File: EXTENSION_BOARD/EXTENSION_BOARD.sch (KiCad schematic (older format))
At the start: 35 parts, among them IC1 TeensyBuffer - 74AHCV541ABQX, IC2 Baro - MS561101BA03-50, J1 EXTIN, J2 BATT, J3 PWM, J4 EXTOUT, U1 Flash - COM-15809, U2 Teensy4.0, U3 MJD148J

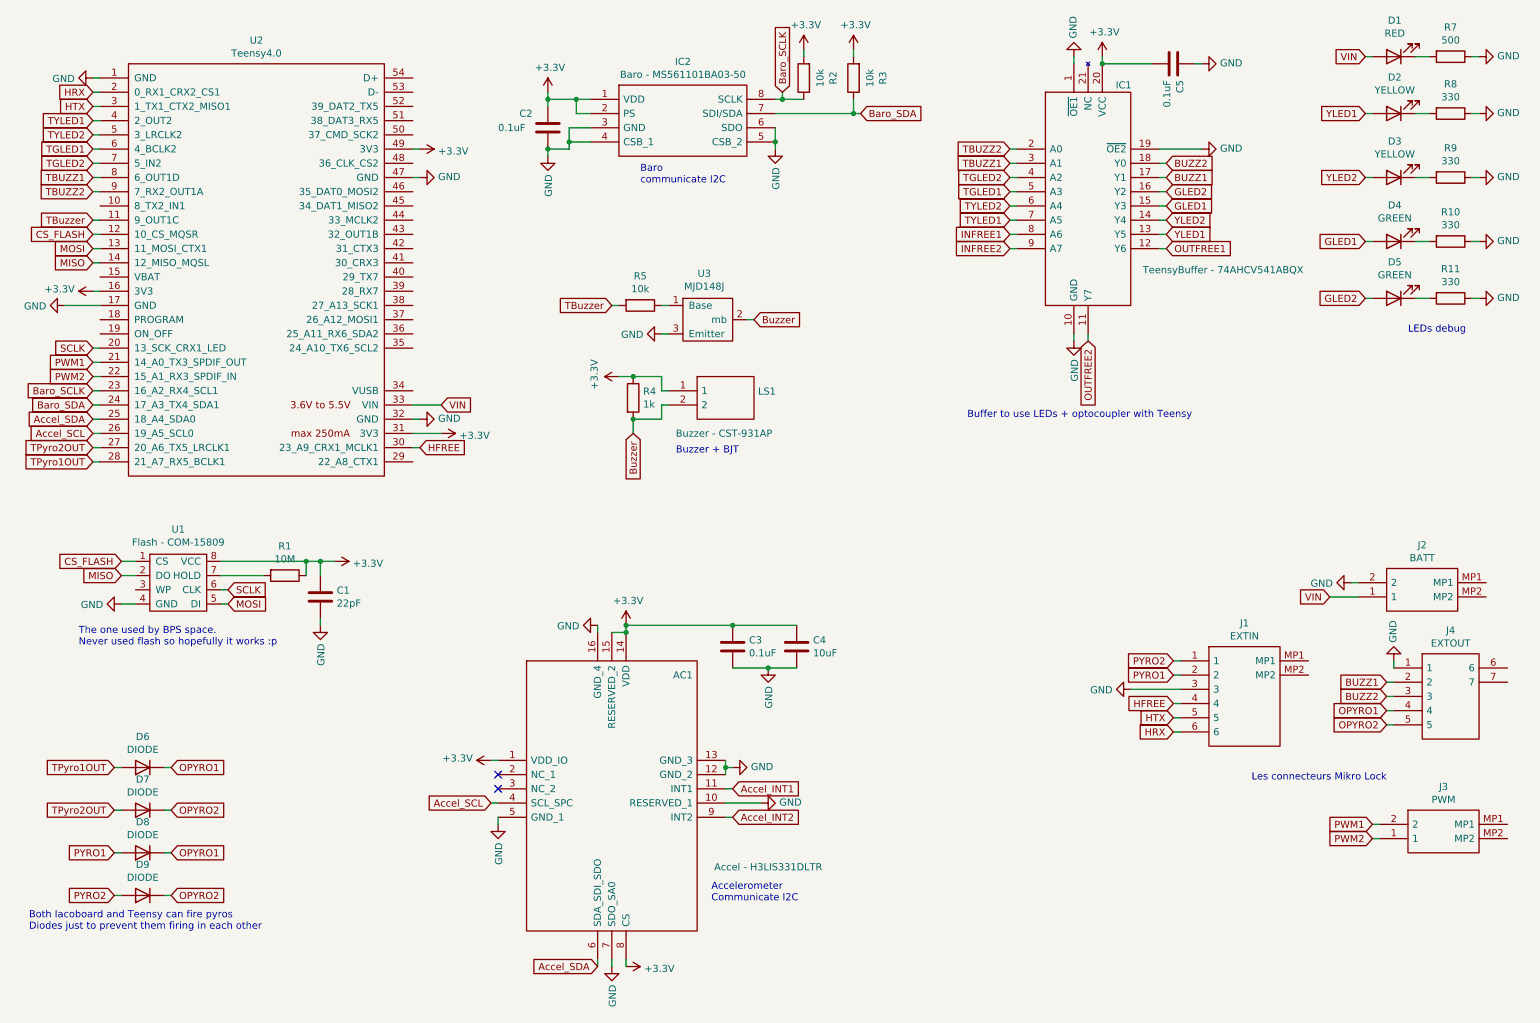
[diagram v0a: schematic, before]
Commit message: t
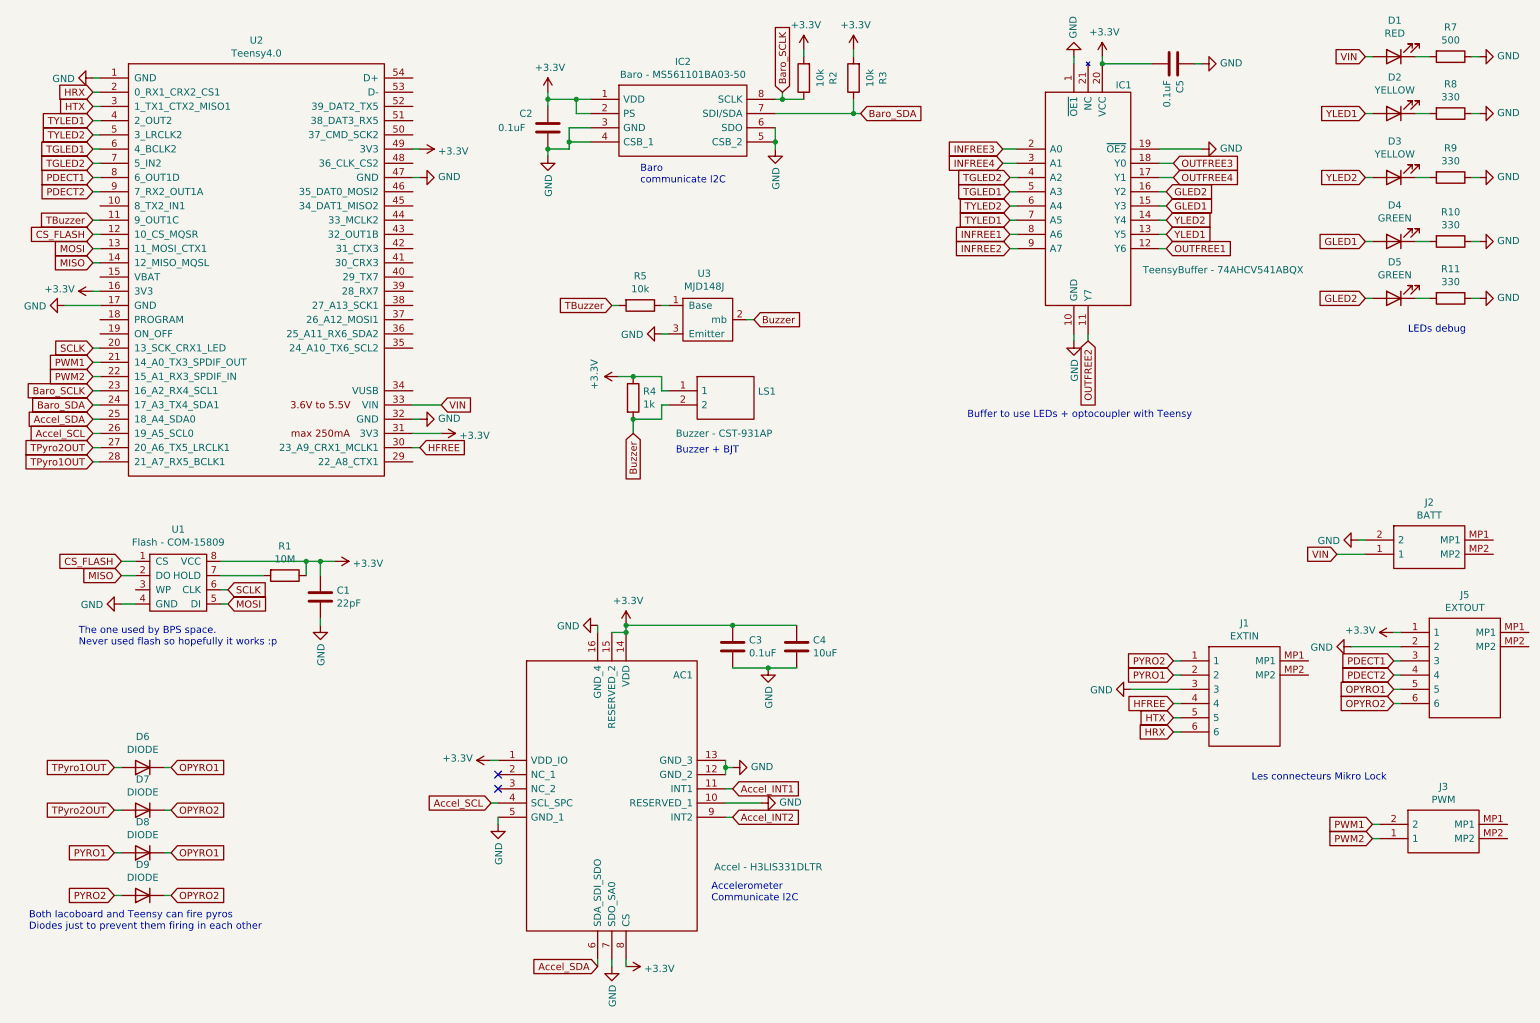
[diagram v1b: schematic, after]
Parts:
- removed J4: EXTOUT, EXTENSION:5055670571, symbol EXTENSION:505567-0571
- added J5: EXTOUT, EXTENSION:5055670671, symbol EXTENSION:505567-0671
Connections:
- net +3V3: now also J5.1
- net GND: now also J5.2
- net OPYRO1: now also J5.5
- net OPYRO2: now also J5.6
- net BUZZ1 renamed OUTFREE4
- net BUZZ2 renamed OUTFREE3
- net TBUZZ1 renamed INFREE4
- net INFREE4: no longer U2.8 (6_OUT1D)
- net TBUZZ2 renamed INFREE3
- net INFREE3: no longer U2.9 (7_RX2_OUT1A)
- new net PDECT1: J5.3, U2.8 (6_OUT1D)
- new net PDECT2: J5.4, U2.9 (7_RX2_OUT1A)
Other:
- moved on the sheet: J2
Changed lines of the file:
@@
 	3500 3450 3300 3450
-$Comp
-L EXTENSION:505567-0571 J4
-U 1 1 618D57EA
-P 10200 5100
-F 0 "J4" H 10600 5365 50  0000 C CNN
-F 1 "EXTOUT" H 10600 5274 50  0000 C CNN
-F 2 "EXTENSION:5055670571" H 10850 5200 50  0001 L CNN
-F 3 "https://www.molex.com/pdm_docs/sd/5055670571_sd.pdf" H 10850 5100 50  0001 L CNN
-F 4 "Molex Micro-Lock PLUS 505567, 1.25mm Pitch, 5 Way, 1 Row, Right Angle PCB Header, Surface Mount" H 10850 5000 50  0001 L CNN "Description"
-F 5 "3" H 10850 4900 50  0001 L CNN "Height"
-F 6 "538-505567-0571" H 10850 4800 50  0001 L CNN "Mouser Part Number"
-F 7 "https://www.mouser.co.uk/ProductDetail/Molex/505567-0571?qs=gt1LBUVyoHnJxHrzoS78pw%3D%3D" H 10850 4700 50  0001 L CNN "Mouser Price/Stock"
-F 8 "Molex" H 10850 4600 50  0001 L CNN "Manufacturer_Name"
-F 9 "505567-0571" H 10850 4500 50  0001 L CNN "Manufacturer_Part_Number"
-	1    10200 5100
-	1    0    0    -1
-$EndComp
 $Comp
 L EXTENSION:505567-0281 J3
@@
 	10050 6300 10100 6300
 $Comp
-L power:GND #PWR034
-U 1 1 618E3668
-P 10200 5050
-F 0 "#PWR034" H 10200 4800 50  0001 C CNN
-F 1 "GND" V 10205 4922 50  0000 R CNN
-F 2 "" H 10200 5050 50  0001 C CNN
-F 3 "" H 10200 5050 50  0001 C CNN
-	1    10200 5050
-	-1   0    0    1
-$EndComp
-Wire Wire Line
-	10150 5500 10200 5500
-Text GLabel 10150 5300 0    50   Input ~ 0
-BUZZ2
-Wire Wire Line
-	10150 5400 10200 5400
-Text GLabel 10150 5200 0    50   Input ~ 0
-BUZZ1
-Text GLabel 10150 5500 0    50   Input ~ 0
-OPYRO2
-Text GLabel 10150 5400 0    50   Input ~ 0
-OPYRO1
-Wire Wire Line
-	10150 5200 10200 5200
-Wire Wire Line
-	10150 5300 10200 5300
-$Comp
 L EXTENSION:505567-0281 J2
 U 1 1 61906994
-P 9950 4500
-F 0 "J2" H 10400 4765 50  0000 C CNN
-F 1 "BATT" H 10400 4674 50  0000 C CNN
-F 2 "EXTENSION:5055670281" H 10700 4600 50  0001 L CNN
-F 3 "https://www.molex.com/pdm_docs/sd/5055670281_sd.pdf" H 10700 4500 50  0001 L CNN
-F 4 "Headers & Wire Housings MicroLockPlus 1.25MM RA HDR SR 2P BLK GLD" H 10700 4400 50  0001 L CNN "Description"
-F 5 "3.9" H 10700 4300 50  0001 L CNN "Height"
-F 6 "538-505567-0281" H 10700 4200 50  0001 L CNN "Mouser Part Number"
-F 7 "https://www.mouser.co.uk/ProductDetail/Molex/505567-0281?qs=gt1LBUVyoHmc7tfcrPDm5A%3D%3D" H 10700 4100 50  0001 L CNN "Mouser Price/Stock"
-F 8 "Molex" H 10700 4000 50  0001 L CNN "Manufacturer_Name"
-F 9 "505567-0281" H 10700 3900 50  0001 L CNN "Manufacturer_Part_Number"
-	1    9950 4500
-	1    0    0    -1
-$EndComp
-Text GLabel 9750 4600 0    50   Input ~ 0
+P 10000 4200
+F 0 "J2" H 10450 4465 50  0000 C CNN
+F 1 "BATT" H 10450 4374 50  0000 C CNN
+F 2 "EXTENSION:5055670281" H 10750 4300 50  0001 L CNN
+F 3 "https://www.molex.com/pdm_docs/sd/5055670281_sd.pdf" H 10750 4200 50  0001 L CNN
+F 4 "Headers & Wire Housings MicroLockPlus 1.25MM RA HDR SR 2P BLK GLD" H 10750 4100 50  0001 L CNN "Description"
+F 5 "3.9" H 10750 4000 50  0001 L CNN "Height"
+F 6 "538-505567-0281" H 10750 3900 50  0001 L CNN "Mouser Part Number"
+F 7 "https://www.mouser.co.uk/ProductDetail/Molex/505567-0281?qs=gt1LBUVyoHmc7tfcrPDm5A%3D%3D" H 10750 3800 50  0001 L CNN "Mouser Price/Stock"
+F 8 "Molex" H 10750 3700 50  0001 L CNN "Manufacturer_Name"
+F 9 "505567-0281" H 10750 3600 50  0001 L CNN "Manufacturer_Part_Number"
+	1    10000 4200
+	1    0    0    -1
+$EndComp
+Text GLabel 9800 4300 0    50   Input ~ 0
 VIN
 Wire Wire Line
-	9900 4500 9950 4500
+	9950 4200 10000 4200
 $Comp
 L power:GND #PWR033
 U 1 1 6190D110
-P 9900 4500
-F 0 "#PWR033" H 9900 4250 50  0001 C CNN
-F 1 "GND" V 9905 4372 50  0000 R CNN
-F 2 "" H 9900 4500 50  0001 C CNN
-F 3 "" H 9900 4500 50  0001 C CNN
-	1    9900 4500
-	0    1    1    0
-$EndComp
-Wire Wire Line
-	9750 4600 9950 4600
+P 9950 4200
+F 0 "#PWR033" H 9950 3950 50  0001 C CNN
+F 1 "GND" V 9955 4072 50  0000 R CNN
+F 2 "" H 9950 4200 50  0001 C CNN
+F 3 "" H 9950 4200 50  0001 C CNN
+	1    9950 4200
+	0    1    1    0
+$EndComp
+Wire Wire Line
+	9800 4300 10000 4300
 $Comp
 L EXTENSION:74AHCV541ABQX IC1
@@
 Text GLabel 8600 2050 2    50   Input ~ 0
 YLED1
-Wire Wire Line
-	8600 1550 8550 1550
 Text GLabel 8600 1950 2    50   Input ~ 0
 YLED2
@@
 GLED2
 Wire Wire Line
-	8600 1650 8550 1650
-Wire Wire Line
 	8600 1750 8550 1750
 Wire Wire Line
 	8600 1850 8550 1850
-Text GLabel 8600 1650 2    50   Input ~ 0
-BUZZ1
-Text GLabel 8600 1550 2    50   Input ~ 0
-BUZZ2
 Wire Wire Line
 	8600 2050 8550 2050
@@
 Wire Wire Line
 	8150 800  8150 850
-Text GLabel 7500 1550 0    50   Input ~ 0
-TBUZZ1
-Text GLabel 7500 1450 0    50   Input ~ 0
-TBUZZ2
 Wire Wire Line
 	7500 1950 7550 1950
@@
 Wire Wire Line
 	7500 1650 7550 1650
-Wire Wire Line
-	7500 1550 7550 1550
-Wire Wire Line
-	7500 1450 7550 1450
 $Comp
 L power:GND #PWR022
@@
 	1050 3050 1100 3050
 Wire Wire Line
-	10200 5050 10200 5100
-Wire Wire Line
 	8350 5250 8700 5250
 Wire Wire Line
@@
 VIN
 Text GLabel 1050 1650 0    50   Input ~ 0
-TBUZZ1
-Text GLabel 1050 1750 0    50   Input ~ 0
-TBUZZ2
+PDECT1
 Wire Wire Line
 	1050 1750 1100 1750
@@
 Text Notes 5400 6750 0    50   ~ 0
 Accelerometer\nCommunicate I2C\n
+Text GLabel 7450 1450 0    50   Input ~ 0
+INFREE3
+Wire Wire Line
+	7450 1450 7550 1450
+Text GLabel 7450 1550 0    50   Input ~ 0
+INFREE4
+Wire Wire Line
+	7450 1550 7550 1550
+Text GLabel 8650 1550 2    50   Input ~ 0
+OUTFREE3
+Text GLabel 8650 1650 2    50   Input ~ 0
+OUTFREE4
+Wire Wire Line
+	8550 1550 8650 1550
+Wire Wire Line
+	8550 1650 8650 1650
+Text GLabel 1050 1750 0    50   Input ~ 0
+PDECT2
+$Comp
+L EXTENSION:505567-0671 J5
+U 1 1 61AEC270
+P 10250 4850
+F 0 "J5" H 10700 5115 50  0000 C CNN
+F 1 "EXTOUT" H 10700 5024 50  0000 C CNN
+F 2 "EXTENSION:5055670671" H 11000 4950 50  0001 L CNN
+F 3 "https://componentsearchengine.com/Datasheets/1/505567-0671.pdf" H 11000 4850 50  0001 L CNN
+F 4 "Molex Micro-Lock PLUS 505567, 1.25mm Pitch, 6 Way, 1 Row, Right Angle PCB Header, Surface Mount" H 11000 4750 50  0001 L CNN "Description"
+F 5 "4.2" H 11000 4650 50  0001 L CNN "Height"
+F 6 "538-505567-0671" H 11000 4550 50  0001 L CNN "Mouser Part Number"
+F 7 "https://www.mouser.co.uk/ProductDetail/Molex/505567-0671?qs=gt1LBUVyoHmQuimOt9l14w%3D%3D" H 11000 4450 50  0001 L CNN "Mouser Price/Stock"
+F 8 "Molex" H 11000 4350 50  0001 L CNN "Manufacturer_Name"
+F 9 "505567-0671" H 11000 4250 50  0001 L CNN "Manufacturer_Part_Number"
+	1    10250 4850
+	1    0    0    -1
+$EndComp
+$Comp
+L power:GND #PWR0101
+U 1 1 61AED9C0
+P 9900 4950
+F 0 "#PWR0101" H 9900 4700 50  0001 C CNN
+F 1 "GND" V 9905 4822 50  0000 R CNN
+F 2 "" H 9900 4950 50  0001 C CNN
+F 3 "" H 9900 4950 50  0001 C CNN
+	1    9900 4950
+	0    1    1    0
+$EndComp
+Text GLabel 10200 5050 0    50   Input ~ 0
+PDECT1
+Text GLabel 10200 5150 0    50   Input ~ 0
+PDECT2
+Text GLabel 10200 5250 0    50   Input ~ 0
+OPYRO1
+Text GLabel 10200 5350 0    50   Input ~ 0
+OPYRO2
+Wire Wire Line
+	10200 5250 10250 5250
+Wire Wire Line
+	10200 5150 10250 5150
+Wire Wire Line
+	10200 5050 10250 5050
+$Comp
+L power:+3.3V #PWR0102
+U 1 1 61B21118
+P 10200 4850
+F 0 "#PWR0102" H 10200 4700 50  0001 C CNN
+F 1 "+3.3V" V 10215 4978 50  0000 L CNN
+F 2 "" H 10200 4850 50  0001 C CNN
+F 3 "" H 10200 4850 50  0001 C CNN
+	1    10200 4850
+	0    -1   -1   0
+$EndComp
+Wire Wire Line
+	9900 4950 10250 4950
+Wire Wire Line
+	10200 4850 10250 4850
+Wire Wire Line
+	10200 5350 10250 5350
 $EndSCHEMATC

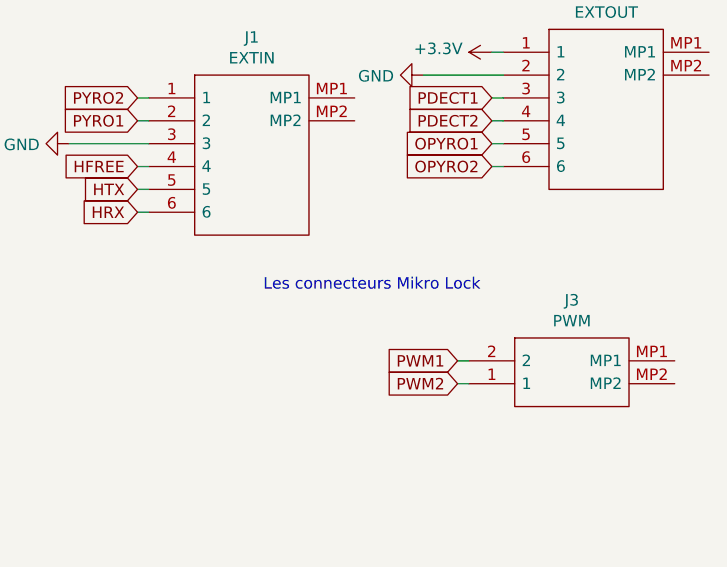
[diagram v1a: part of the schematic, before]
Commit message: a
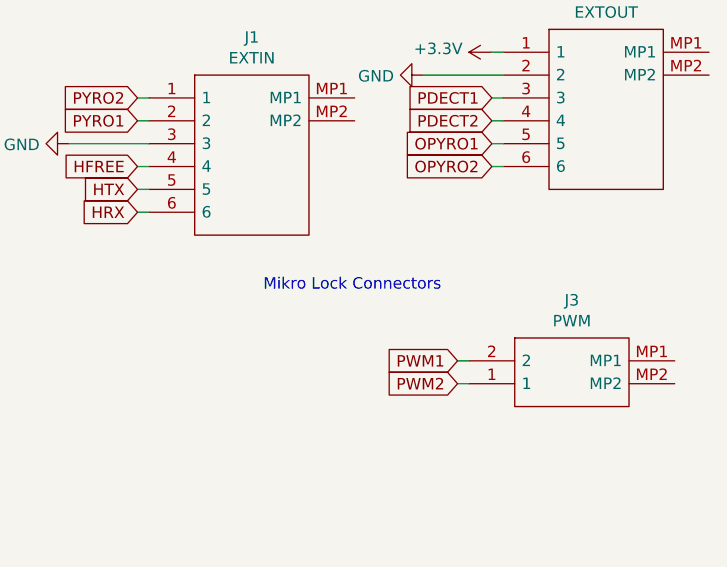
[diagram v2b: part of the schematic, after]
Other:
- note added: "Mikro Lock Connectors\n"
- note removed: "Les connecteurs Mikro Lock"
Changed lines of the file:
@@
 Both Iacoboard and Teensy can fire pyros\nDiodes just to prevent them firing in each other
 Text Notes 9200 5900 0    50   ~ 0
-Les connecteurs Mikro Lock
+Mikro Lock Connectors\n
 Text Notes 10300 2750 0    50   ~ 0
 LEDs debug
